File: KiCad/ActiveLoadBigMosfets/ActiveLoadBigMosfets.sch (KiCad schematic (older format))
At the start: 106 parts

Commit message: More PCB work
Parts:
- removed C? (x3): 10u/X7R/100V, symbol Device:C
- removed C?: 10u, symbol Device:C
- removed J?: FanOut, symbol Connector_Generic:Conn_01x03
- removed Q?: IRLML2244, Package_TO_SOT_SMD:SOT-23, symbol Transistor_FET:IRLML5203
- removed SW?: Rotary_Encoder_Switch, symbol Device:Rotary_Encoder_Switch
- removed U? (x3): TLV2372, symbol Amplifier_Operational:TLV2372
- added C13: 63SXV33M, Capacitor_SMD:CP_Elec_8x11.9, symbol Device:CP
- added C14: 4u7/16V/85mR, Capacitor_SMD:C_0805_2012Metric, symbol Device:C
- added C15: 10n, Capacitor_SMD:C_0805_2012Metric, symbol Device:C
- added C22, C48: 6TPE150MF, Capacitor_Tantalum_SMD:CP_EIA-7343-31_Kemet-D, symbol Device:CP
- added C31, C33, C35: 10u, Capacitor_SMD:C_0805_2012Metric, symbol Device:C
- added C34, C36, C49: 100n, Capacitor_SMD:C_0805_2012Metric, symbol Device:C
- added C40, C41, C42, C43, C44: 1n, Capacitor_SMD:C_0805_2012Metric, symbol Device:C
- added C50: 10u/10V, Capacitor_SMD:C_0805_2012Metric, symbol Device:C
- added F1: 10A, JPFuses:Fuseholder5x20_horiz_open_inline_Type-I, symbol Device:Fuse
- added FL1, FL2: BNX025, Filter:Filter_Murata_BNX025, symbol Filter:BNX025
- added H1, H2, H3, H4: MountingHole, MountingHole:MountingHole_3.2mm_M3, symbol Mechanical:MountingHole
- added J6: FanOut, Connector:FanPinHeader_1x04_P2.54mm_Vertical, symbol Connector_Generic:Conn_01x04
- added J7: PowerInput2, JPConnectors:SolderingHoles-2_P6.00mm_D2.0mm, symbol Connector_Generic:Conn_01x02
- added J8: PowerInput3, JPConnectors:SolderingHoles-2_P6.00mm_D2.0mm, symbol Connector_Generic:Conn_01x02
- added J9: PowerInput4, JPConnectors:SolderingHoles-2_P6.00mm_D2.0mm, symbol Connector_Generic:Conn_01x02
- added Q1: IRLML2502, Package_TO_SOT_SMD:SOT-23, symbol Transistor_FET:IRLML2060
- added Q10, Q11, Q12, Q13, Q14: IXFK44N50P, Package_TO_SOT_THT:TO-264-3_Vertical, symbol Device:Q_NMOS_GDS
- added R13: 100k, Resistor_SMD:R_0805_2012Metric, symbol Device:R
- added R27, R28, R29, R30, R32, R39, R40, R41, R42, R44, R64, R65: 10k, Resistor_SMD:R_0805_2012Metric, symbol Device:R
- added R33, R34, R35, R36, R37: 15k, Resistor_SMD:R_0805_2012Metric, symbol Device:R
- added R45, R46, R49, R50, R55: 0R1, Resistor_SMD:R_2512_6332Metric, symbol Device:R
- added R53, R54, R56, R57, R61: 1k, Resistor_SMD:R_0805_2012Metric, symbol Device:R
- added R63: 20m, Resistor_SMD:R_2512_6332Metric, symbol Device:R
- added R66, R67, R68, R69: 10, Resistor_SMD:R_0805_2012Metric, symbol Device:R
- added R70: 5k, Resistor_SMD:R_0805_2012Metric, symbol Device:R
- added RV1: 5k, Potentiometer_SMD:Potentiometer_ACP_CA6-VSMD_Vertical, symbol Device:R_POT
- added SW1: Rotary_Encoder_Switch, Rotary_Encoder:RotaryEncoder_Alps_EC11E-Switch_Vertical_H20mm_CircularMountingHoles, symbol Device:Rotary_Encoder_Switch
- added SW2: SW_Push, Button_Switch_SMD:SW_SPST_EVQP0, symbol Switch:SW_Push
- added U5, U6, U7: TLV2374, Package_SO:SOIC-14_3.9x8.7mm_P1.27mm, symbol myLib:TLV2374
- C1, C10, C16, C17, C18, C19, C2, C20, C21, C23, C24, C25, C26, C3, C30, C32, C37, C38, C39, C4, C45, C46, C47, C5, C6, C7, C8, C9: renamed from C?; footprint (none) -> Capacitor_SMD:C_0805_2012Metric
- C11, C12: renamed from C?; footprint (none) -> Capacitor_Tantalum_SMD:CP_EIA-7343-31_Kemet-D
- C27, C28: renamed from C?; value 10u/16V/85mR -> 4u7/16V/85mR; footprint (none) -> Capacitor_SMD:C_0805_2012Metric
- C29: renamed from C?; footprint (none) -> Capacitor_SMD:CP_Elec_6.3x7.7
- D1, D2: renamed from D?; footprint (none) -> Diode_SMD:D_SMB
- D3: renamed from D?; footprint (none) -> Diode_SMD:D_MiniMELF
- D4: renamed from D?; footprint (none) -> LED_SMD:LED_0805_2012Metric
- J1: renamed from J?; footprint (none) -> Connector_FFC-FPC:TE_0-1734839-6_1x06-1MP_P0.5mm_Horizontal
- J2: renamed from J?; footprint (none) -> JPConnectors:SolderingHoles-2_P6.00mm_D2.0mm
- J3: renamed from J?; footprint (none) -> Connector_PinHeader_2.54mm:PinHeader_1x06_P2.54mm_Vertical
- J4: renamed from J?; footprint (none) -> JPConnectors:Hirose_FH12-50S-0.5SH_1x50-1MP_P0.50mm_Horizontal
- J5: renamed from J?; footprint (none) -> Connector_PinHeader_2.54mm:PinHeader_2x10_P2.54mm_Vertical_SMD
- L1: renamed from L?; footprint (none) -> Inductor_SMD:L_0805_2012Metric
- L2: renamed from L?; footprint (none) -> JPInductors:L_Wuerth_WE-HCF
- L3: renamed from L?; value L -> 7447714330; footprint (none) -> Inductor_SMD:L_Wuerth_WE-PDF
- Q9: renamed from Q?; footprint (none) -> Package_TO_SOT_THT:TO-264-3_Vertical
- R1: renamed from R?; value R -> 20m; footprint (none) -> Resistor_SMD:R_2512_6332Metric
- R10, R12, R15, R16, R17, R18, R19, R2, R20, R21, R22, R24, R26, R38, R47, R48, R51, R52, R58, R59, R60, R62, R7, R8: renamed from R?; footprint (none) -> Resistor_SMD:R_0805_2012Metric
- R11: renamed from R?; value 133k -> 30k; footprint (none) -> Resistor_SMD:R_0805_2012Metric
- R14: renamed from R?; value 10k2 -> 15k4; footprint (none) -> Resistor_SMD:R_0805_2012Metric
- R23: renamed from R?; value 86k6 -> 100k; footprint (none) -> Resistor_SMD:R_0805_2012Metric
- R25: renamed from R?; value 10k -> 11k; footprint (none) -> Resistor_SMD:R_0805_2012Metric
- R3, R6: renamed from R?; footprint (none) -> Jumper:SolderJumper-2_P1.3mm_Bridged_RoundedPad1.0x1.5mm
- R31: renamed from R?; value 10k -> 15k; footprint (none) -> Resistor_SMD:R_0805_2012Metric
- R4, R5: renamed from R?; footprint (none) -> Jumper:SolderJumper-2_P1.3mm_Open_RoundedPad1.0x1.5mm
- R43: renamed from R?; footprint (none) -> Resistor_SMD:R_2512_6332Metric
- R9: renamed from R?; value 44k2 -> 68k; footprint (none) -> Resistor_SMD:R_0805_2012Metric
- U1: renamed from U?; footprint (none) -> Package_SO:SOIC-8-1EP_3.9x4.9mm_P1.27mm_EP2.41x3.3mm_ThermalVias
- U2: renamed from U?; footprint (none) -> Package_TO_SOT_SMD:SOT-223-3_TabPin2
- U4: renamed from U?; value LM2735XMF -> LM2735YMF
- U8: renamed from U?; footprint (none) -> Package_TO_SOT_THT:TO-220-5_Vertical
- Y1: renamed from Y?; footprint (none) -> Crystal:Crystal_SMD_5032-2Pin_5.0x3.2mm
- gave numbers to parts that had none: 9
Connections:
- net GNDPWR is gone; now on net GND: D1.2 (A), J2.1 (Pin_1), R43.2
- net +12V: now also C31.1, C33.1, C34.1, C35.1, C36.1, FL2.2 (CB), R70.1, U5.4 (V+), U6.4 (V+), U7.4 (V+); no longer C26.1, C27.1, C28.1, C29.1, D2.1 (K), R23.2
- net +3V3: now also C22.1, C49.1, R64.1, R66.2, R67.2, R68.2, R69.2; no longer R2.2
- net +4V: now also C48.1, C50.1, FL1.2 (CB); no longer C10.1, C11.1, C12.1, L2.2, R9.1
- net DisplayLEDCtrl: now also Q1.1 (G)
- net Enc_A: now also U3.22 (PA6); no longer U3.58 (PB6)
- net Enc_B: now also U3.23 (PA7); no longer U3.59 (PB7)
- net Enc_Switch: now also U3.41 (PA8); no longer U3.61 (PB8)
- net FanPWD: now also U3.21 (PA5), J6.4 (Pin_4); no longer Q8.1 (G), U3.22 (PA6)
- net FanSensor: now also U3.27 (PB1), J6.3 (Pin_3); no longer U3.23 (PA7)
- net GND: now also U1.7 (GND), U1.9 (PowerPAD), C13.2, FL1.3 (PSG), J7.1 (Pin_1), J8.1 (Pin_1), J9.1 (Pin_1), R13.2, R45.2, R46.2, R49.2, R50.2, R55.2; no longer C1.2, C17.2, C18.2, C19.2, C2.2, C20.2, C21.2, C23.2, C24.2, C25.1, C27.2, C28.2, C29.2, C3.2, C30.2, C32.2, C37.2, C38.2, C4.2, C45.2, C46.2, C47.2, C5.2, C6.2, C7.1, D3.2 (A), D4.1 (K), J1.6 (Pin_6), J3.3 (Pin_3), J4.1 (Pin_1), J4.11 (Pin_11), J4.12 (Pin_12), J4.13 (Pin_13), J4.14 (Pin_14), J4.34 (Pin_34), J4.43 (Pin_43), J4.48 (Pin_48), J4.49 (Pin_49), J4.50 (Pin_50), J4.8 (Pin_8), J4.9 (Pin_9), J5.10 (Pin_10), J5.12 (Pin_12), J5.14 (Pin_14), J5.16 (Pin_16), J5.18 (Pin_18), J5.20 (Pin_20), J5.4 (Pin_4), J5.6 (Pin_6), J5.8 (Pin_8), Q4.2 (S), Q5.2 (S), Q6.2 (S), Q7.2 (S), R11.2, R16.2, R17.2, R18.2, R19.2, R21.1, R25.1, R48.2, R5.2, R6.2, U2.2 (GND), U3.12 (VSSA), U3.18 (VSS), U3.31 (VSS), U3.47 (VSS), U3.60 (BOOT0), U3.63 (VSS), U4.2 (GND), U8.3 (GND), U9.1 (A1), U9.2 (A0), U9.7 (GND)
- net LCD_D_C: now also U3.59 (PB7)
- net LCD_RDX: now also U3.57 (PB5)
- net LCD_RESET: now also U3.50 (PA15)
- net LCD_SELECT: now also U3.61 (PB8)
- net LCD_WRX: now also U3.58 (PB6)
- net LED: now also U3.33 (PB12); no longer U3.50 (PA15)
- net LoadLevel: now also RV1.2, U5.10 (+), U5.5 (+), U6.10 (+), U6.5 (+), U7.10 (+), U7.5 (+)
- net PowerIn+: now also F1.1, R63.2; no longer J2.2 (Pin_2)
- net PowerIn-: now also U1.2 (Vin), U1.3 (EN), C13.1, Q10.2 (D), Q11.2 (D), Q12.2 (D), Q13.2 (D), Q14.2 (D), R63.1
- net at C39.2, Q9.1 (G): now also U5.7
- net at C39.1, R26.2: now also U5.6 (-)
- net at R38.2: now also U5.3 (+)
- net at R31.1, R48.1: now also U5.2 (-)
- net at R26.1, R31.2: now also U5.1
- net at D3.1 (K), Q8.2 (S): now also J6.2 (Pin_2)
- net at U1.1 (Boot): now also C8.2
- net at U1.4 (RT_SYNC): now also R11.1
- net at U1.5 (FB): now also C10.2, R14.1, R9.2
- net at U1.6 (SS): now also C16.1
- net at U1.8 (SW): now also C8.1, D1.1 (K), L2.2
- net Switch: now reaches U3.42 (PA9)
- net Switch: now also C15.1, R65.1
- net FanPower: now reaches U3.45 (PA12)
- net FanPower: now also Q8.1 (G)
- net GNDD: now reaches R20.1, R22.1
- net GNDD: now also C1.2, C17.2, C18.2, C19.2, C2.2, C20.2, C21.2, C23.2, C24.2, C25.1, C27.2, C28.2, C29.2, C3.2, C30.2, C37.2, C38.2, C4.2, C45.2, C46.2, C47.2, C5.2, C6.2, C7.1, D4.1 (K), J1.6 (Pin_6), J3.3 (Pin_3), J4.11 (Pin_11), J4.12 (Pin_12), J4.13 (Pin_13), J4.14 (Pin_14), J4.34 (Pin_34), J4.43 (Pin_43), J4.48 (Pin_48), J4.49 (Pin_49), J4.50 (Pin_50), J4.8 (Pin_8), J4.9 (Pin_9), J5.10 (Pin_10), J5.12 (Pin_12), J5.14 (Pin_14), J5.16 (Pin_16), J5.18 (Pin_18), J5.20 (Pin_20), J5.4 (Pin_4), J5.6 (Pin_6), J5.8 (Pin_8), Q4.2 (S), Q5.2 (S), Q6.2 (S), Q7.2 (S), R16.2, R17.2, R18.2, R19.2, R2.2, R21.1, R25.1, R5.2, R6.2, U2.2 (GND), U3.12 (VSSA), U3.18 (VSS), U3.31 (VSS), U3.47 (VSS), U3.60 (BOOT0), U3.63 (VSS), U4.2 (GND), U8.3 (GND), U9.1 (A1), U9.2 (A0), U9.7 (GND), C14.2, C15.2, C22.2, C48.2, C49.2, C50.2, FL1.4 (CG), FL2.3 (PSG), Q1.2 (S), RV1.3, SW1.C, SW1.S2, SW2.1
- net at R52.2, R58.1: now also SW1.B
- net at R51.2, R62.1: now also SW1.A
- net at R47.2, R59.2: now also SW1.S1
- new net: F1.2, J2.2 (Pin_2), J7.2 (Pin_2), J8.2 (Pin_2), J9.2 (Pin_2)
- new net: C14.1, C26.1, C27.1, C28.1, C29.1, D2.1 (K), FL2.1 (B), R23.2
- new net: R11.2, R13.1
- new net: C10.1, C11.1, C12.1, FL1.1 (B), L2.1, R9.1
- new net: J4.1 (Pin_1), Q1.3 (D)
- new net: J4.2 (Pin_2), R66.1
- new net: J4.3 (Pin_3), R67.1
- new net: J4.4 (Pin_4), R68.1
- new net: J4.5 (Pin_5), R69.1
- new net: R70.2, RV1.1
- new net: C40.2, Q10.1 (G), U5.8
- new net: C40.1, R27.2, U5.9 (-)
- new net: R39.2, U5.12 (+)
- new net: R33.1, R53.1, U5.13 (-)
- new net: R27.1, R33.2, U5.14
- new net: Q10.3 (S), R39.1, R45.1
- new net: C41.2, Q11.1 (G), U6.7
- new net: Q11.3 (S), R40.1, R46.1
- new net: R34.1, R54.1, U6.2 (-)
- new net: R40.2, U6.3 (+)
- new net: R28.1, R34.2, U6.1
- new net: C41.1, R28.2, U6.6 (-)
- new net: C42.2, Q12.1 (G), U6.8
- new net: C42.1, R29.2, U6.9 (-)
- new net: R41.2, U6.12 (+)
- new net: R35.1, R56.1, U6.13 (-)
- new net: R29.1, R35.2, U6.14
- new net: Q12.3 (S), R41.1, R49.1
- new net: C43.2, Q13.1 (G), U7.7
- new net: Q13.3 (S), R42.1, R50.1
- new net: R36.1, R57.1, U7.2 (-)
- new net: R42.2, U7.3 (+)
- new net: R30.1, R36.2, U7.1
- new net: C43.1, R30.2, U7.6 (-)
- new net: C44.2, Q14.1 (G), U7.8
- new net: C44.1, R32.2, U7.9 (-)
- new net: R44.2, U7.12 (+)
- new net: R37.1, R61.1, U7.13 (-)
- new net: R32.1, R37.2, U7.14
- new net: Q14.3 (S), R44.1, R55.1
- new net: R64.2, R65.2, SW2.2
- new net GNDA: C31.2, C32.2, C33.2, C34.2, C35.2, C36.2, D3.2 (A), FL2.4 (CG), J6.1 (Pin_1), R48.2, R53.2, R54.2, R56.2, R57.2, R61.2, U5.11 (V-), U6.11 (V-), U7.11 (V-)
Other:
- note added: "G=15"
- note added: "Rthjc=0.2Ohm\nRthcs=1Ohm\nRthsa=0.5Ohm\nRth=1.7Ohm\n(125-40)/1.7=50W\n\nRth=0.25+0+0.5=0.75 Ohm\n85/0.75=114W"
- note added: "Vo=12.665V"
- note added: "Vo=4.062V"
- note added: "https://webench.ti.com/power-designer/switching-regulator/customize/8?AppType=None&Flavor=NA&O1I=1.5&O1V=4&Topology=BUCK&VinMax=30.00&VinMin=5&VoltageOption=NA&base_pn=LMR14020S&flavor=NA&lang_chosen=en_US&op_TA=30&optfactor=3&origin=pf_panel\nhttps://webench.ti.com/power-designer/switching-regulator/customize/7?AppType=None&Flavor=None&O1I=0.4&O1V=12&Topology=Boost&VinMax=4&VinMin=4&VoltageOptio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"
- note removed: "G=10"
- note removed: "Rthjc=0.25Ohm\nRthcs=1Ohm\nRthsa=0.5Ohm\nRth=1.75Ohm\n\n(125-40)/2.25=48W"
- note removed: "https://webench.ti.com/power-designer/switching-regulator/customize/8?AppType=None&Flavor=NA&O1I=1.5&O1V=4&Topology=BUCK&VinMax=30.00&VinMin=5&VoltageOption=NA&base_pn=LMR14020S&flavor=NA&lang_chosen=en_US&op_TA=30&optfactor=3&origin=pf_panel"
- moved on the sheet: C1, C10, C11, C12, C16, C19, C20, C21, C23, C24, C25, C26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

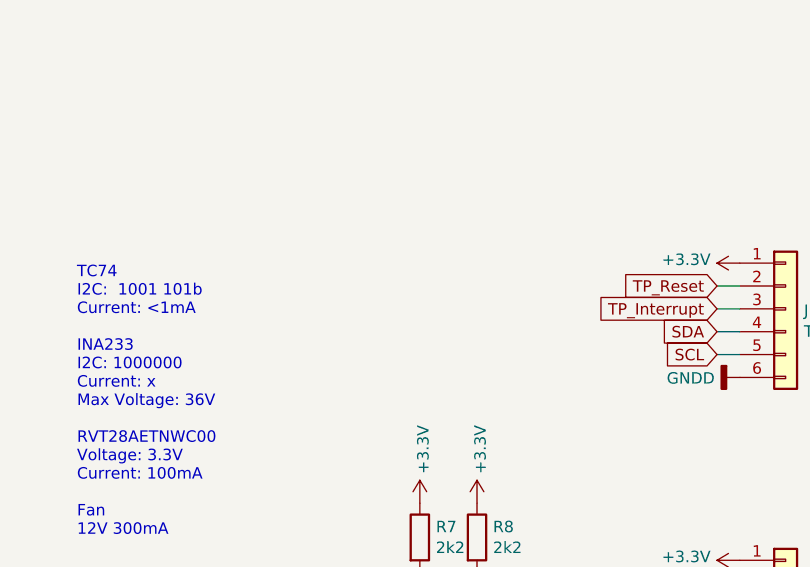
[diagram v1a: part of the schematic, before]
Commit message: More pcb work
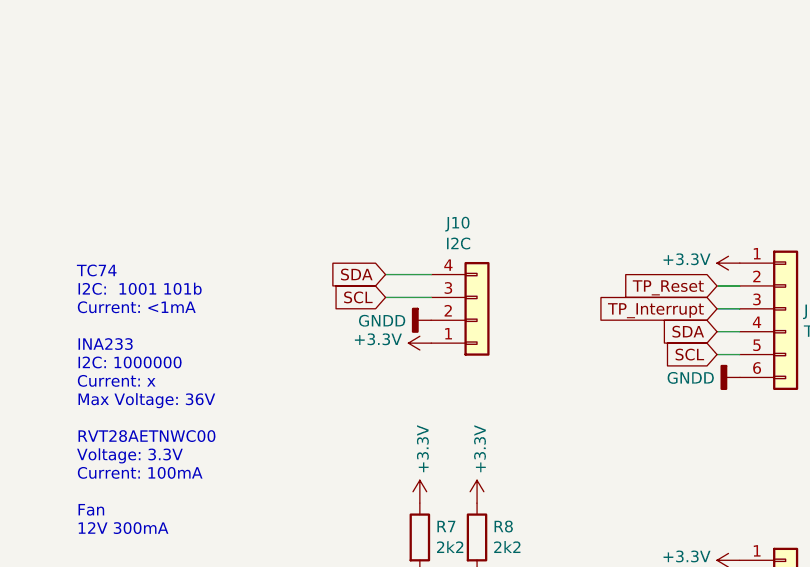
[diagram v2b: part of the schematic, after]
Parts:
- added J10: I2C, Connector_PinHeader_2.54mm:PinHeader_1x04_P2.54mm_Vertical, symbol Connector_Generic:Conn_01x04
- C2, C20, C21, C23, C24, C25, C3, C32, C34, C36, C37, C38, C4, C49, C5, C7, C8, C9: footprint Capacitor_SMD:C_0805_2012Metric -> Capacitor_SMD:C_0603_1608Metric
- FL1, FL2: footprint Filter:Filter_Murata_BNX025 -> JPInductors:Filter_Murata_BNX025
- L3: footprint Inductor_SMD:L_Wuerth_WE-PDF -> JPInductors:L_Wuerth_WE-PDF_Handsoldering
- R1, R43, R45, R46, R49, R50, R55, R63: footprint Resistor_SMD:R_2512_6332Metric -> Resistor_SMD:R_2512_6332Metric_Pad1.52x3.35mm_HandSolder
- R10, R12, R20, R21, R22, R24, R26, R27, R28, R29, R30, R32, R38, R39, R40, R41, R42, R44, R47, R51, R52, R58, R59, R60, R62, R64, R65: footprint Resistor_SMD:R_0805_2012Metric -> Resistor_SMD:R_0603_1608Metric
- U4: footprint Package_TO_SOT_SMD:SOT-23-5 -> Package_TO_SOT_SMD:SOT-23-5_HandSoldering
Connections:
- net +3V3: now also J10.1 (Pin_1)
- net GNDD: now also J10.2 (Pin_2)
- net SCL: now also J10.3 (Pin_3)
- net SDA: now also J10.4 (Pin_4)

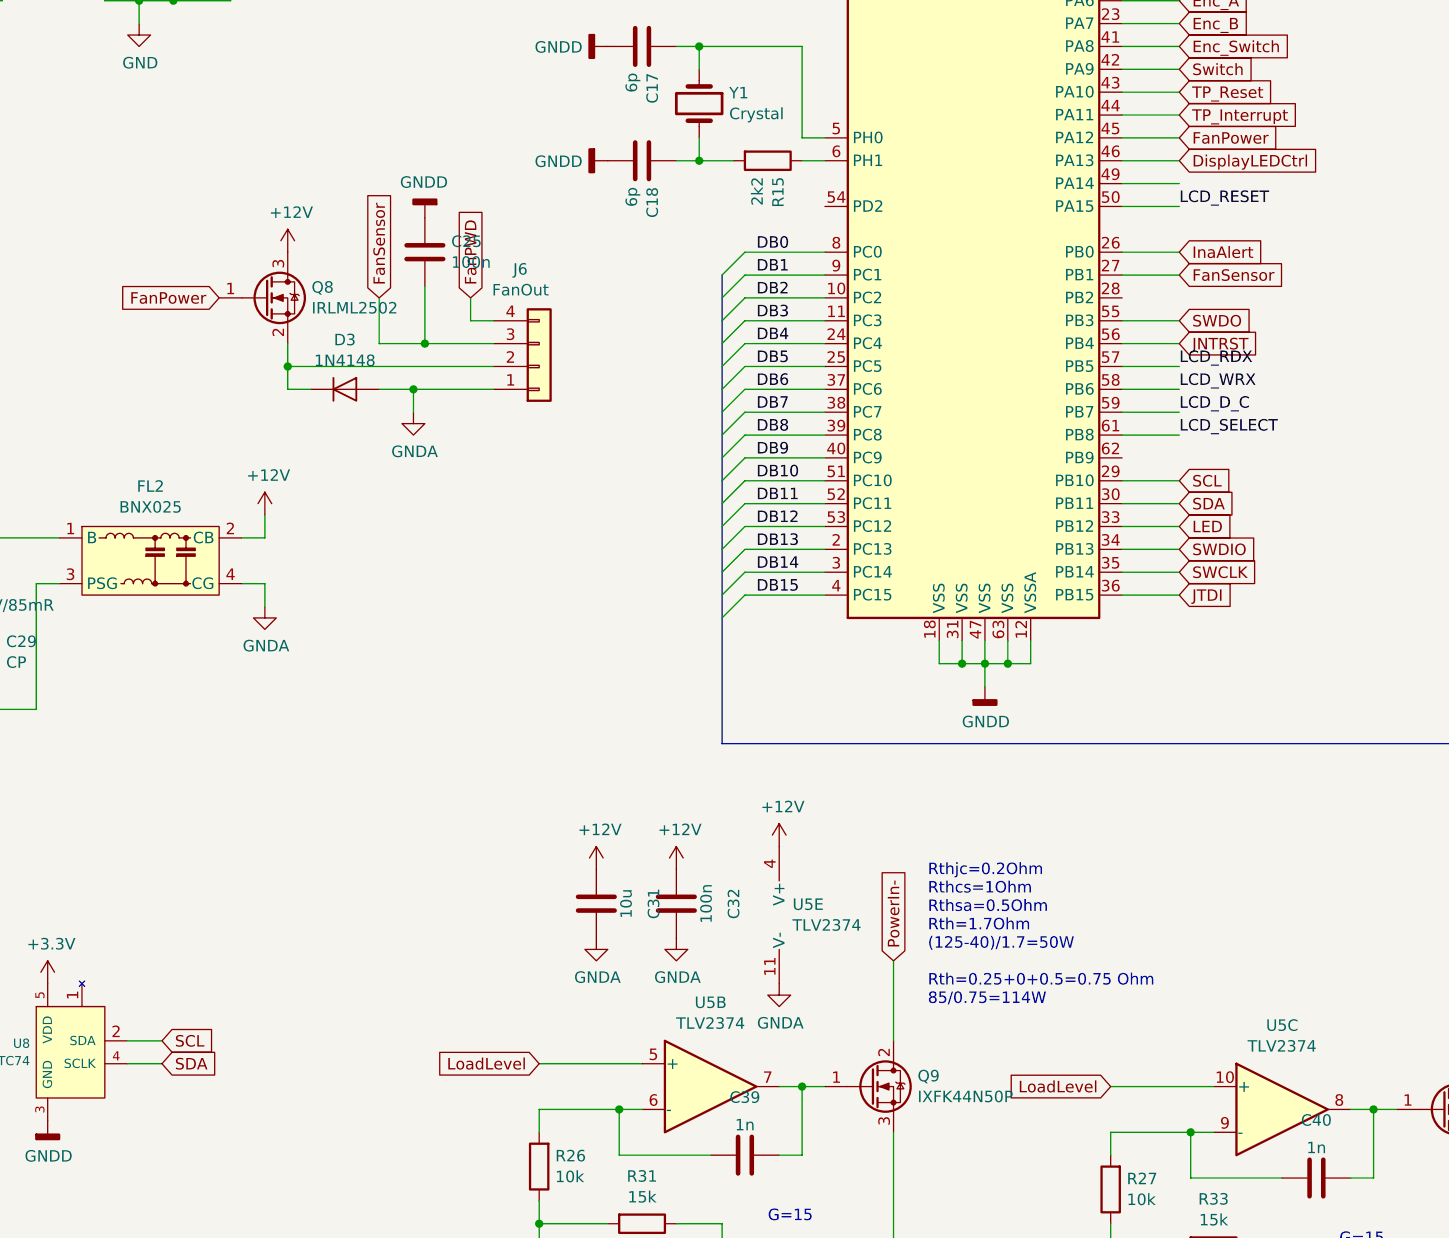
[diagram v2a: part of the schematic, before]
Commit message: PCB work
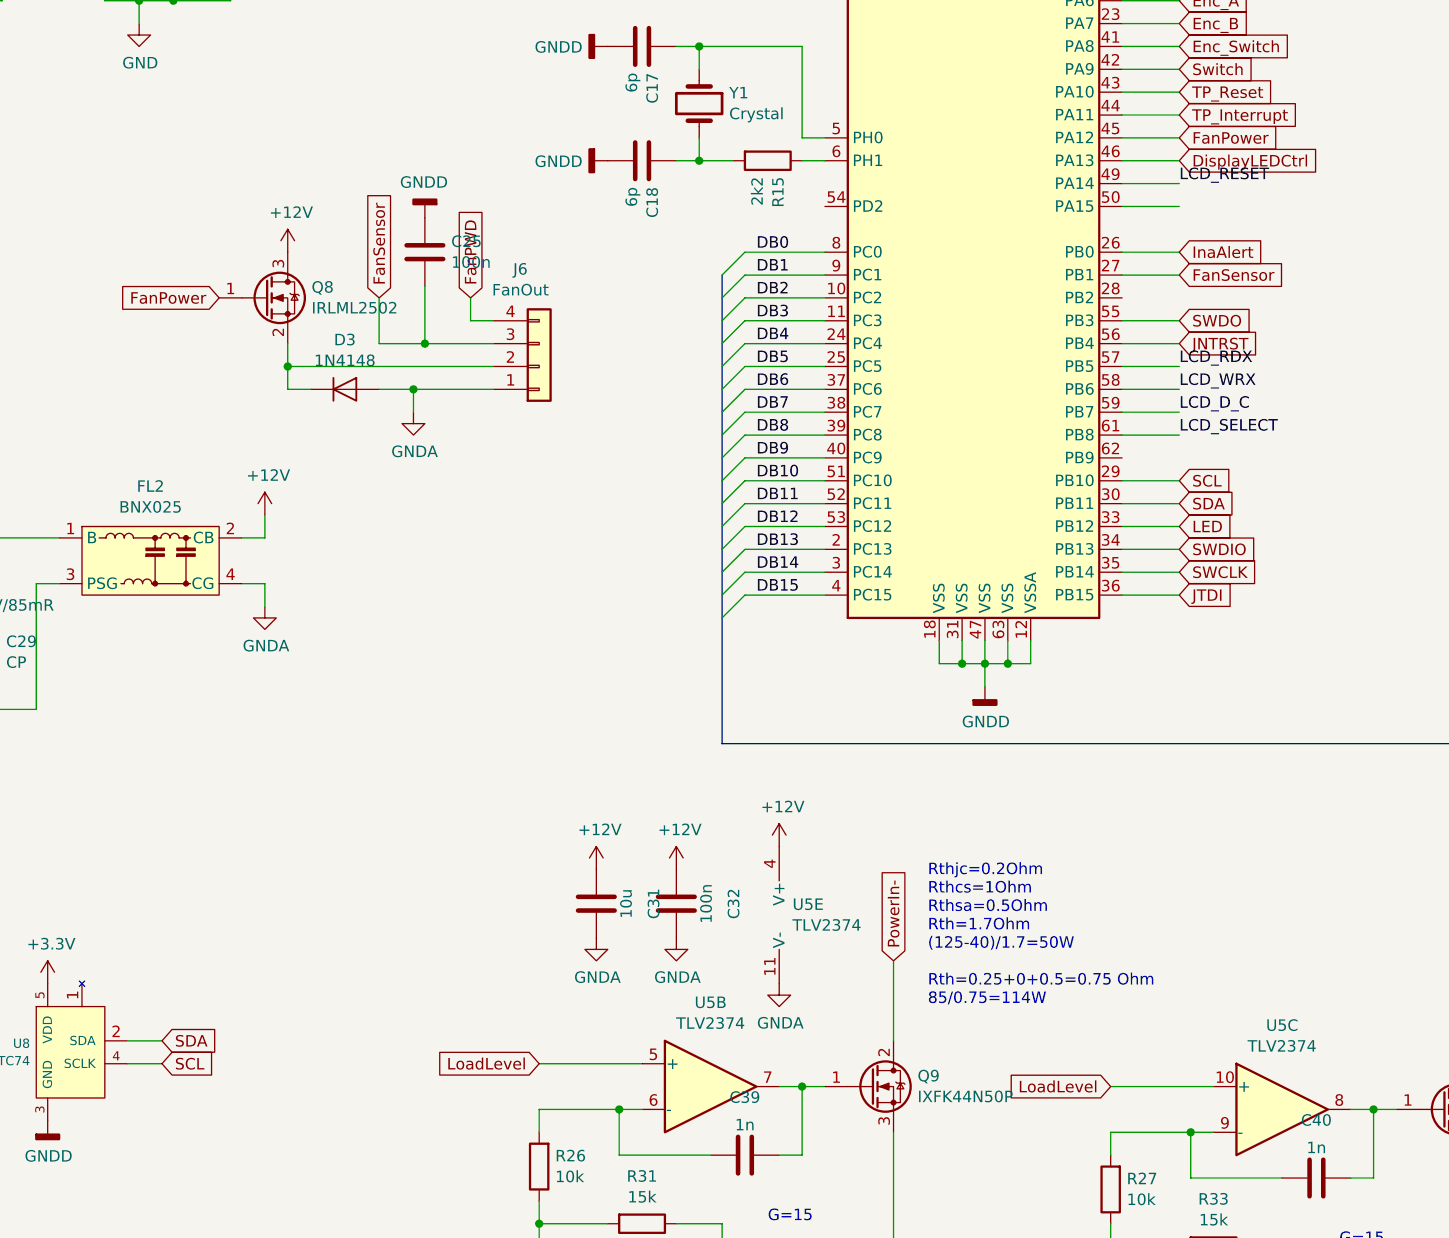
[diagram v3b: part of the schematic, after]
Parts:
- J4: footprint JPConnectors:Hirose_FH12-50S-0.5SH_1x50-1MP_P0.50mm_Horizontal -> JPConnectors:Molex-50S-0.5SH_1x50-P0.50mm_Horizontal
- SW2: footprint Button_Switch_SMD:SW_SPST_EVQP0 -> Button_Switch_SMD:SW_SPST_B3S-1000
- U8: footprint Package_TO_SOT_THT:TO-220-5_Vertical -> Connector_PinHeader_2.54mm:PinHeader_1x05_P2.54mm_Vertical
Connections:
- net LCD_RESET: now also U3.49 (PA14); no longer U3.50 (PA15)
- net SCL: now also U8.4 (SCLK); no longer U8.2 (SDA)
- net SDA: now also U8.2 (SDA); no longer U8.4 (SCLK)
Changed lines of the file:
@@
 F 0 "U8" H 4823 8038 40  0000 R CNN
 F 1 "TC74" H 4823 7962 40  0000 R CNN
-F 2 "Package_TO_SOT_THT:TO-220-5_Vertical" H 4950 8000 60  0001 C CNN
+F 2 "Connector_PinHeader_2.54mm:PinHeader_1x05_P2.54mm_Vertical" H 4950 8000 60  0001 C CNN
 F 3 "" H 4950 8000 60  0000 C CNN
 	1    4950 8000
@@
 	1    0    0    -1
 $EndComp
-Text GLabel 5400 7950 2    50   Input ~ 0
+Text GLabel 5400 8050 2    50   Input ~ 0
 SCL
 Text GLabel 6250 2300 2    50   Input ~ 0
 SCL
-Text GLabel 5400 8050 2    50   Input ~ 0
+Text GLabel 5400 7950 2    50   Input ~ 0
 SDA
 Wire Wire Line
@@
 F 0 "J4" H 12850 4067 50  0000 C CNN
 F 1 "RVT28AETNWC00" H 12850 3976 50  0000 C CNN
-F 2 "JPConnectors:Hirose_FH12-50S-0.5SH_1x50-1MP_P0.50mm_Horizontal" H 12800 2650 50  0001 C CNN
+F 2 "JPConnectors:Molex-50S-0.5SH_1x50-P0.50mm_Horizontal" H 12800 2650 50  0001 C CNN
 F 3 "~" H 12800 2650 50  0001 C CNN
 	1    12800 2650
@@
 Wire Wire Line
 	1000 6000 1000 6150
-Text Label 9850 4300 0    50   ~ 0
+Text Label 9850 4200 0    50   ~ 0
 LCD_RESET
 Wire Wire Line
@@
 F 0 "SW2" H 1700 12285 50  0000 C CNN
 F 1 "SW_Push" H 1700 12194 50  0000 C CNN
-F 2 "Button_Switch_SMD:SW_SPST_EVQP0" H 1700 12200 50  0001 C CNN
+F 2 "Button_Switch_SMD:SW_SPST_B3S-1000" H 1700 12200 50  0001 C CNN
 F 3 "~" H 1700 12200 50  0001 C CNN
 	1    1700 12000
